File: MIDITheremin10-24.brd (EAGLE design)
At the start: 101.6 x 68.6 mm, 102 parts, among them IC1 TL072P, IC2 TL072P, J1 DCJ0202, T1 2N3904, T2 2N3904, T3 2N3904, T4 2N3904, T5 2N3904, T6 2N3904

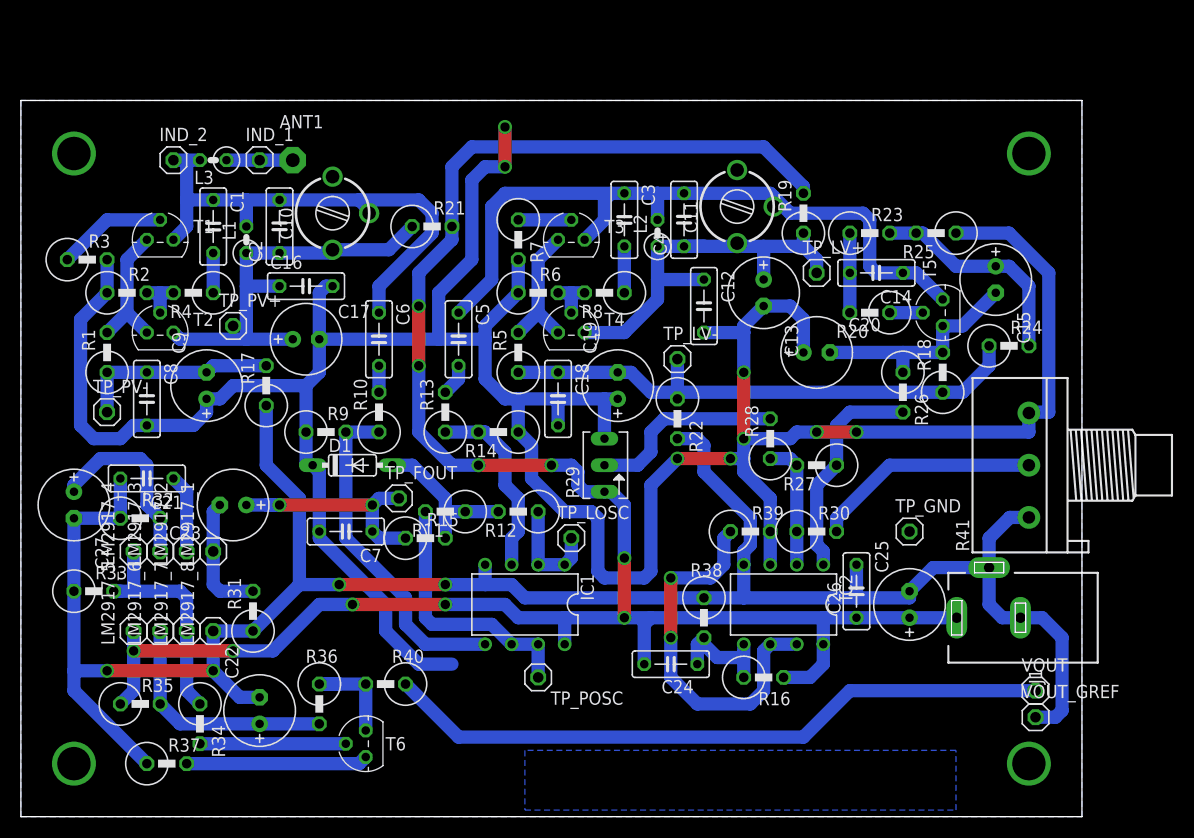
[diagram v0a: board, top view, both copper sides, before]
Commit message: Add files via upload
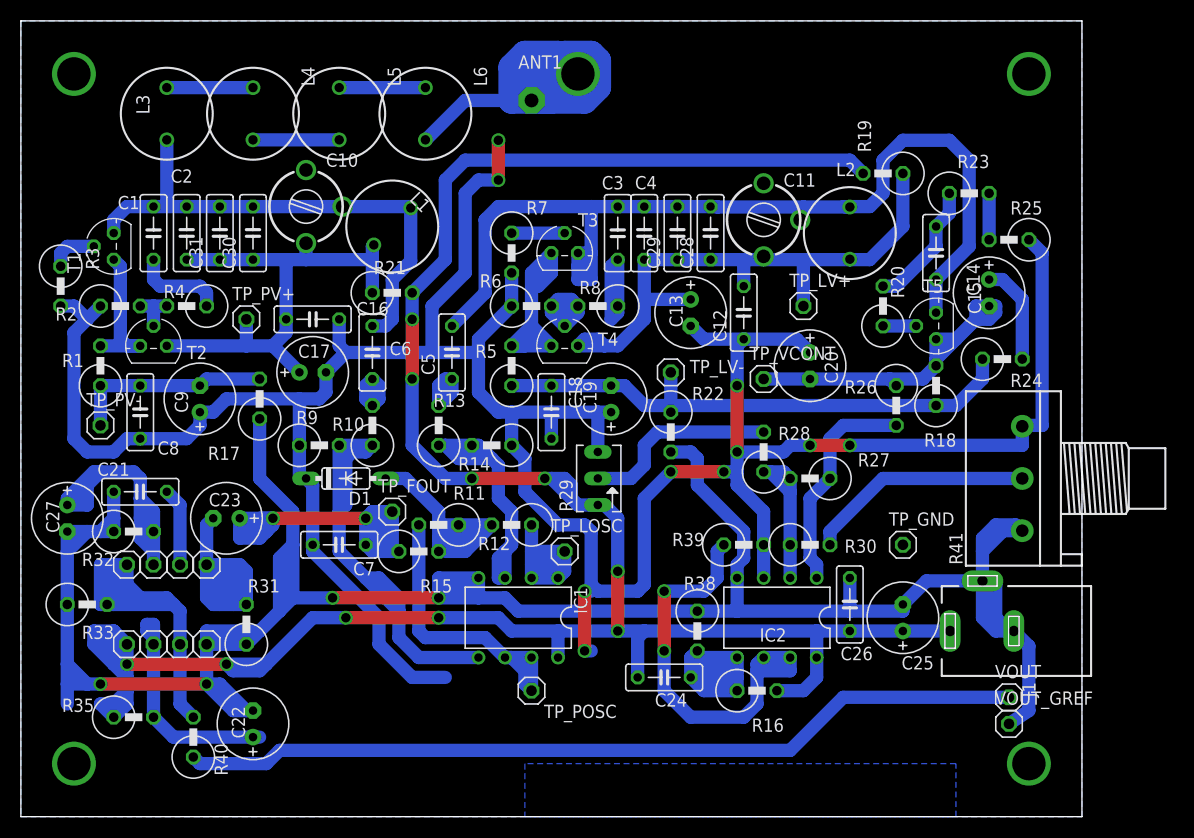
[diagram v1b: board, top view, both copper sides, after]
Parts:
- removed IND_1, IND_2: (no value), pinhead:1X01
- removed R34: 620k, rcl:0411V
- removed R36, R37: 10k, rcl:0411V
- removed T6: 2N3904, transistor-neu-to92:TO92
- added C28, C29, C30, C31: tune, resistor:C050-025X075
- added L4, L5, L6: 10mH, rcl:6000-XXXX-RC
- added TP_VCONT: (no value), pinhead:1X01
- L1, L2: device resistor:0207/2V -> rcl:6000-XXXX-RC
- L3: value 40mH *** -> 10mH; device resistor:0207/2V -> rcl:6000-XXXX-RC
- R27: value 56k -> 51k
- R28: value 33k -> 22k
- moved ANT1 23.6 mm to (48.9, 68.6)
- moved L2 18.4 mm to (79.4, 55.9)
- moved R40 18.3 mm to (16.5, 8.26), turned to 90 degrees
- moved L1 14.0 mm to (35.6, 56.5), turned to 45 degrees
- moved R23 10.3 mm to (91.4, 59.7)
- moved C2 8.91 mm to (15.9, 55.9)
- moved R19 7.67 mm to (81.9, 61.6), turned to 180 degrees
- moved R21 7.41 mm to (36.2, 50.2)
- moved C13 7.24 mm to (64.1, 48.3)
- moved R25 7.01 mm to (94.0, 55.2)
- moved L3 6.29 mm to (14.0, 67.3), turned to 270 degrees
- moved C14 6.02 mm to (87.6, 54.0), turned to 90 degrees
- moved C1 5.75 mm to (12.7, 55.9)
- moved R3 4.49 mm to (3.81, 50.2), turned to 270 degrees
- moved T1 4.49 mm to (8.89, 54.6), turned to 90 degrees
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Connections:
- removed net VOUT: R36.1, R40.2, T6.1
- new net ANT: ANT1.1, L6.2
- net LOCAL_RESONANCE: now also C28.2, C29.2
- net L_OSC_V+: now also C28.1, C29.1
- net N$19: now also L5.1, L6.1; no longer ANT1.1, IND_1.1, L3.1
- net N$28: now also L3.1, L4.1; no longer R34.2, T6.2
- net N$31: no longer R36.2
- net N$35: now also L4.2, L5.2; no longer R37.2, T6.3
- net N$4: now also C30.2, C31.2; no longer IND_2.1
- net N$9: now also TP_VCONT.1
- net NON_INVERT_OUT: now also R40.2; no longer R34.1
- net P_OSC_V+: now also C30.1, C31.1
- net V-: no longer R37.1
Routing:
- net ANT: track 0.00 -> 46.4 mm, vias 0 -> 1
- net V-: track 207.6 -> 241.1 mm
- net V+: track 202.2 -> 234.5 mm
- net LOCAL_RESONANCE: track 71.0 -> 95.4 mm
- net L_OSC_V+: track 42.0 -> 59.1 mm
- net N$38: track 64.3 -> 81.0 mm
- net N$18: track 22.1 -> 38.5 mm
- net NON_INVERT_OUT: track 22.4 -> 37.8 mm
- net N$34: track 12.0 -> 26.2 mm
- net N$33: track 17.7 -> 31.6 mm
- net N$9: track 21.6 -> 35.5 mm
- net N$13: track 32.4 -> 46.0 mm
- net N$36: track 10.9 -> 23.2 mm
- net N$6: track 13.2 -> 24.4 mm
- net VOUT: track 10.8 -> 0.00 mm
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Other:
- board size 101.6 x 68.6 mm -> 101.6 x 76.2 mm
